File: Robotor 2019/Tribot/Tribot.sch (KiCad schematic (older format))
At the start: 85 parts, among them J1 Conn_01x03_Male, J2 Conn_01x04_Female, J3 USB_B_Mini, J4 Conn_01x04_Female, J5 Conn_01x04_Female, J7 Conn_01x03_Female, J8 Conn_01x03_Female, M1 Motor_DC, M2 Motor_DC, U1 AMS1117-3V3, U3 AMS1117-5.0, U4 STM32F103C8Tx, U5 ITR8307, U6 L298P, U7 ITR8307, U8 ITR8307, U9 ITR8307, Y1 32.768Khz, Y2 8Mhz

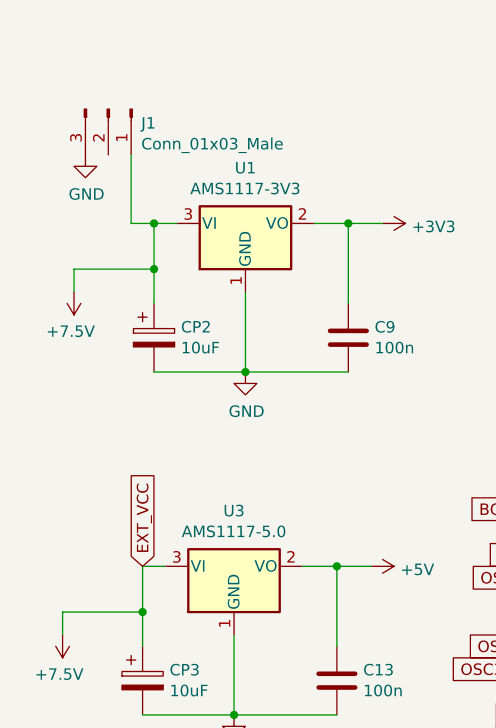
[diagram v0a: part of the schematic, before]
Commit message: Tribot bottom circuit board final version (hopefully)
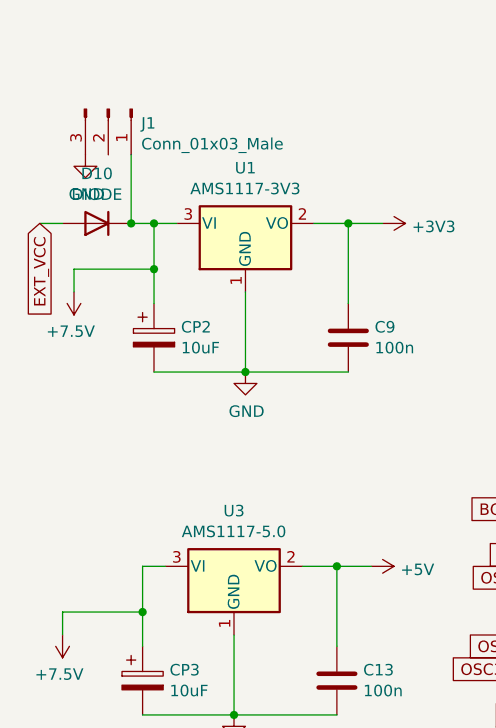
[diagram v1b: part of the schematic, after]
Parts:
- added D10: DIODE, Diode_THT:D_A-405_P5.08mm_Vertical_AnodeUp, symbol Simulation_SPICE:DIODE
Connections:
- net +7.5V: now also D10.2 (K); no longer J3.1 (VBUS)
- new net EXT_VCC: D10.1 (A), J3.1 (VBUS)
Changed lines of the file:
@@
 Text GLabel 6200 1450 2    50   Input ~ 0
 EXT_VCC
-Text GLabel 1100 2800 1    50   Input ~ 0
+Text GLabel 650  1300 3    50   Input ~ 0
 EXT_VCC
 $Comp
@@
 Text GLabel 5750 4000 1    50   Input ~ 0
 M1IN2_B
+$Comp
+L Simulation_SPICE:DIODE D10
+U 1 1 5D3C17DD
+P 900 1300
+F 0 "D10" H 900 1517 50  0000 C CNN
+F 1 "DIODE" H 900 1426 50  0000 C CNN
+F 2 "Diode_THT:D_A-405_P5.08mm_Vertical_AnodeUp" H 900 1300 50  0001 C CNN
+F 3 "~" H 900 1300 50  0001 C CNN
+F 4 "Y" H 900 1300 50  0001 L CNN "Spice_Netlist_Enabled"
+F 5 "V" H 900 1300 50  0001 L CNN "Spice_Primitive"
+	1    900  1300
+	1    0    0    -1
+$EndComp
+Connection ~ 1050 1300
+Wire Wire Line
+	650  1300 750  1300
 $EndSCHEMATC
